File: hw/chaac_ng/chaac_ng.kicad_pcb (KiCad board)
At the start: 4 copper layers, 71 parts, among them J1 Battery, J2 Solar, J3 TC2030-CTX, J4 Conn_01x04, P1 USB_C_Plug_USB2.0, SW1 SW_Push, SW2 SW_Push, U1 E22-X00M22S, U2 BQ24074RGT, U3 TPS76333, U4 MAX3221, U5 STM32L412KBTx, U6 TPS61252DSG, Y1 32.768kHz

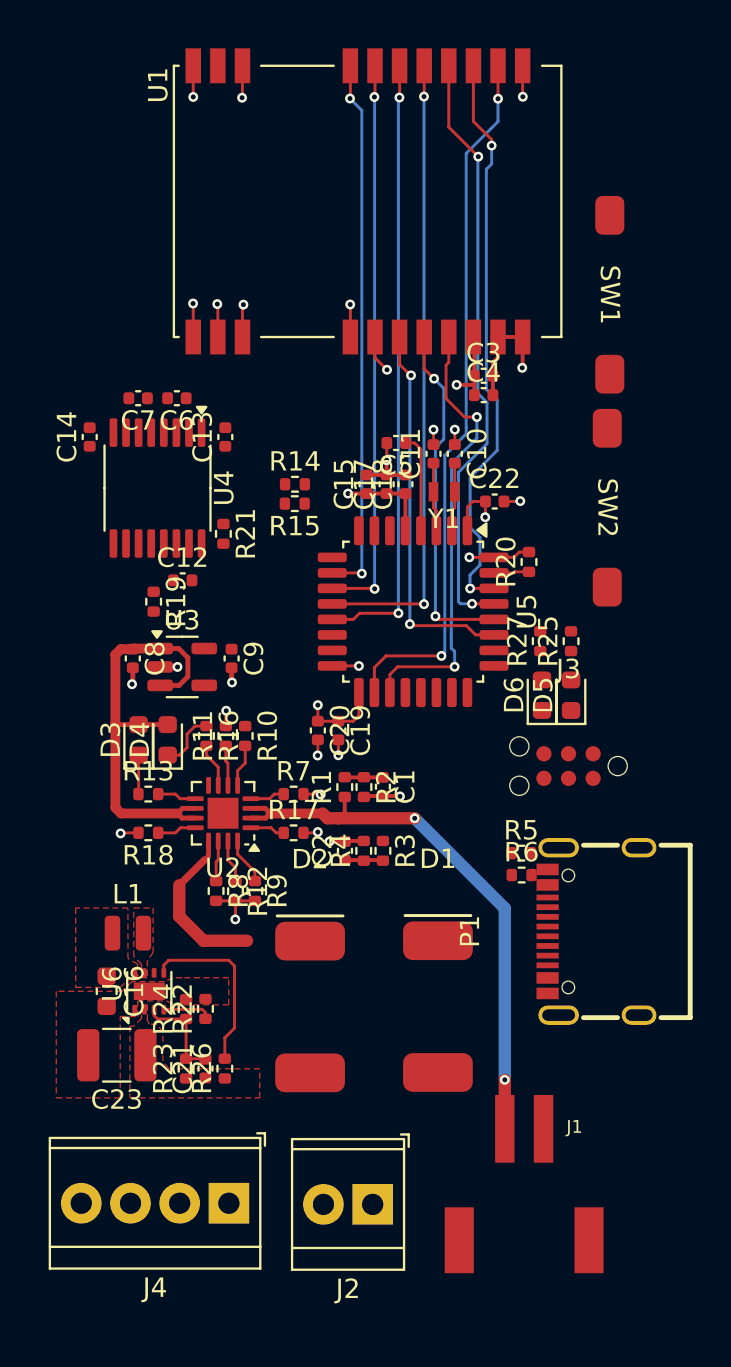
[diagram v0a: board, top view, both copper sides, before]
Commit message: More layout/routing
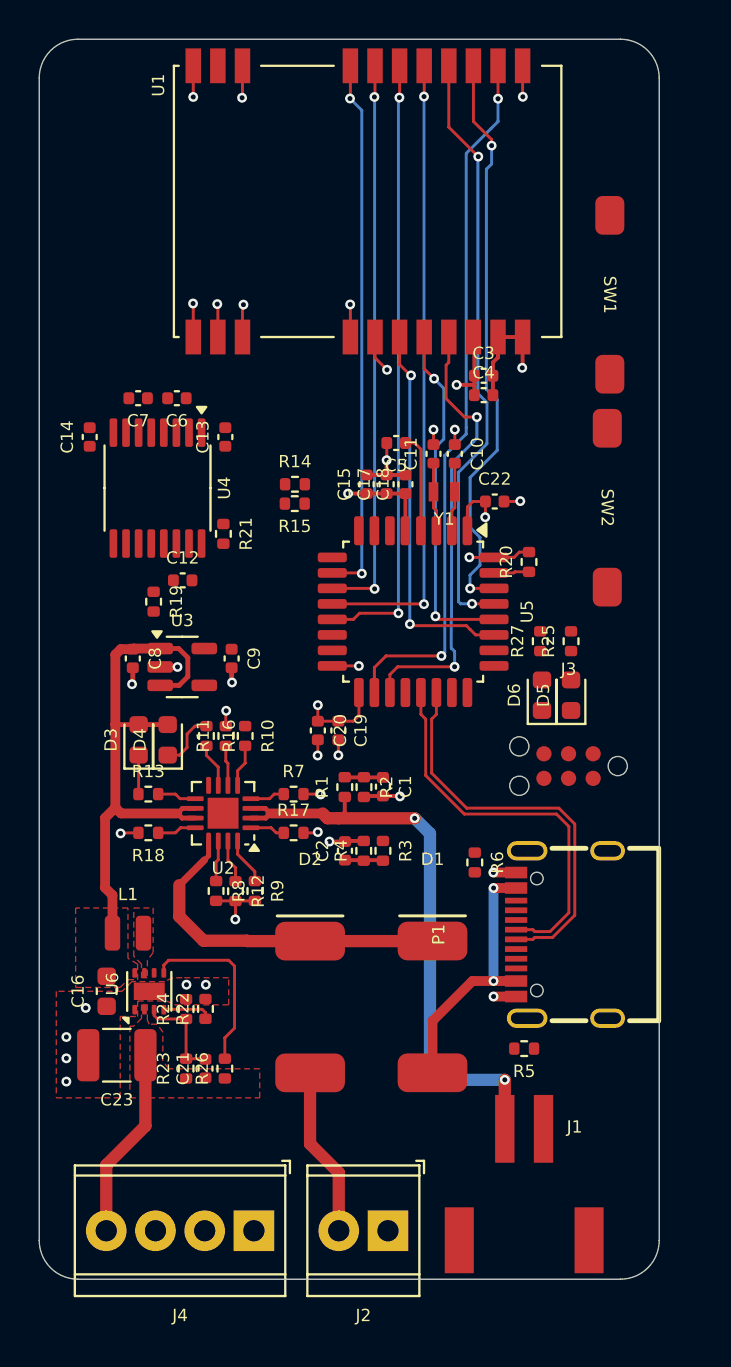
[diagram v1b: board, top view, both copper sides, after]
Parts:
- moved R5 10.1 mm to (106.0, 124.1), turned to 180 degrees
- moved R6 2.51 mm to (103.5, 114.5), turned to -90 degrees
- moved J4 1.92 mm to (92.1, 133.5)
- moved P1 1.63 mm to (108.0, 118.2)
- moved J2 1.57 mm to (99.0, 133.5)
- moved D1 0.28 mm to (101.3, 121.9)
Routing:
- net /USB_DP: track 0.00 -> 21.0 mm
- net /USB_DN: track 0.00 -> 20.5 mm
- net VBUS: track 0.00 -> 13.8 mm, vias 0 -> 2
- net +6V: track 0.00 -> 9.90 mm
- net Net-(D1-K): track 8.54 -> 18.1 mm
- net /SOLAR_IN: track 0.00 -> 8.76 mm
- net /VIN: track 22.6 -> 29.5 mm
- net GND: track 44.4 -> 46.7 mm, vias 27 -> 35
- net /VBATT: track 29.0 -> 30.7 mm
- added copper zone on In1.Cu, net GND
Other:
- board outline added: 32 x 64 mm
